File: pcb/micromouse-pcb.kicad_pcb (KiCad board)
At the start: 4 copper layers, 120 x 80 mm, 52 parts, among them J1 Conn_01x08, J1_MotorEncoder1 Conn_01x06, J2_MotorEncoder1 Conn_01x06, J3 Conn_01x08, J4 Conn_01x08, Q1 BS170, Q2 TEFT4300, Q3 BS170, Q4 TEFT4300, Q5 BS170, Q6 TEFT4300, Q7 BS170, Q8 TEFT4300, SW1 SW_SPDT, U1 Teensy_4.1, U2 L7805

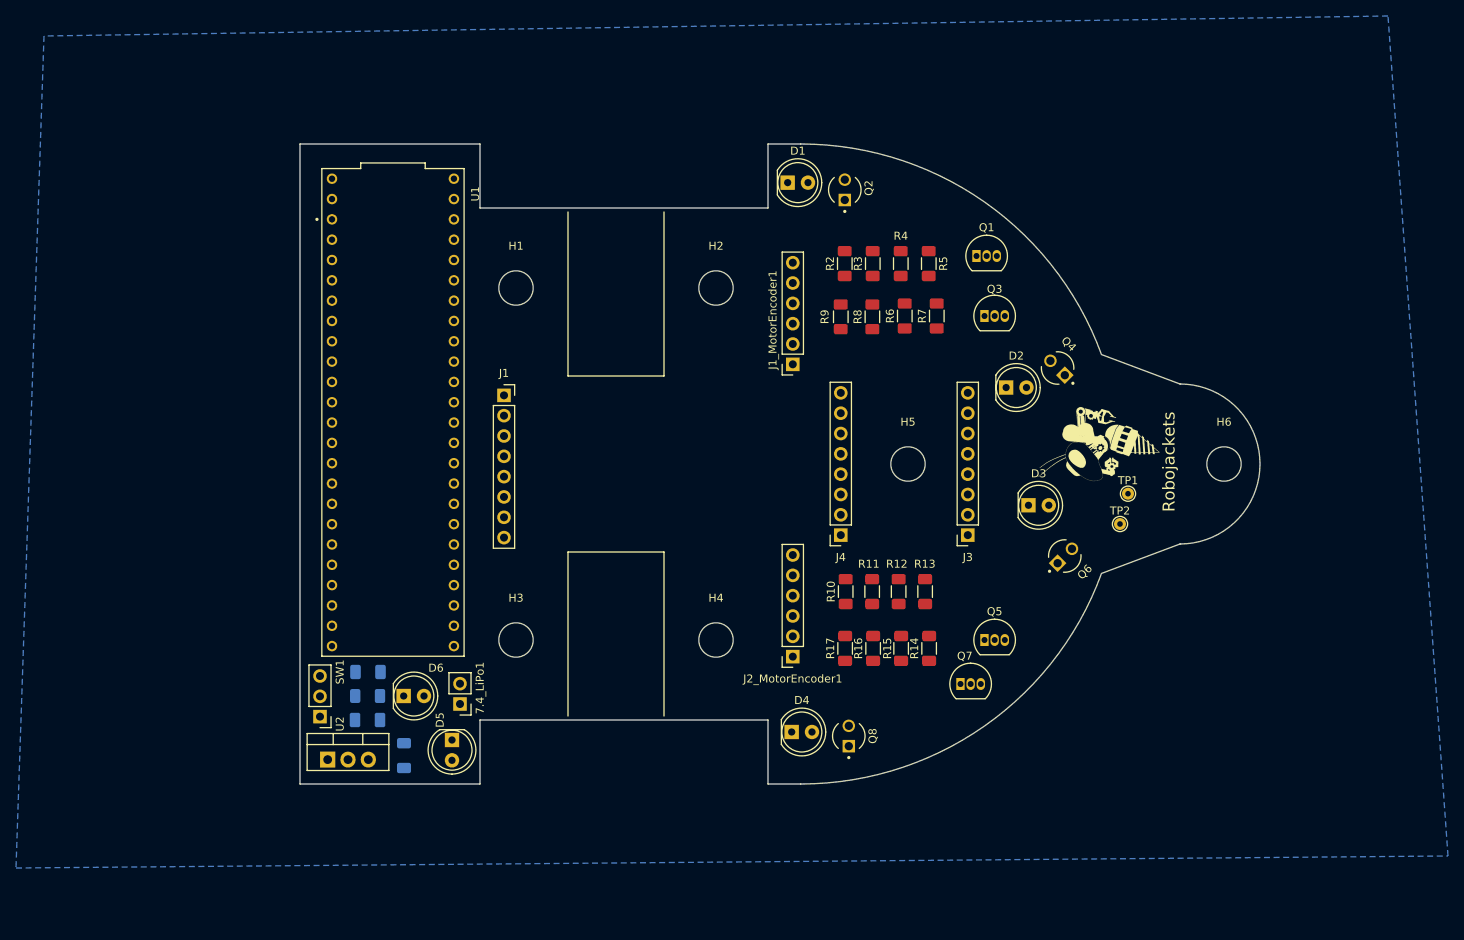
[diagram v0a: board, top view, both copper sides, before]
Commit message: Done placement
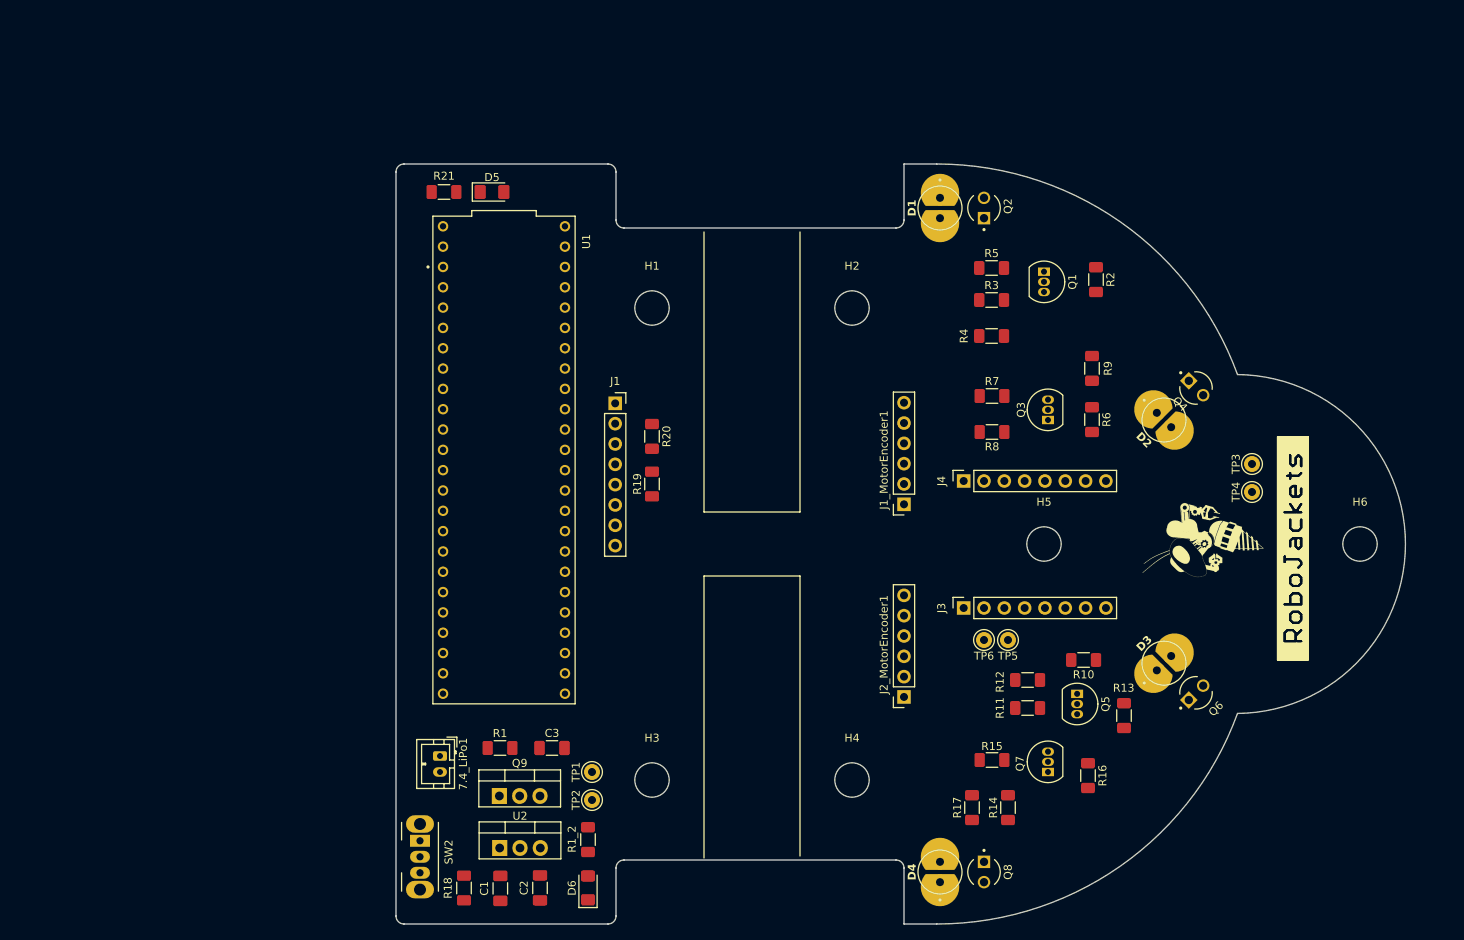
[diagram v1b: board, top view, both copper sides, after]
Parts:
- removed the ? at (122.5, 53.6)
- removed R1_1: R_US, Resistor_SMD:R_1206_3216Metric_Pad1.30x1.75mm_HandSolder
- removed SW1: SW_SPDT, Connector_PinHeader_2.54mm:PinHeader_1x03_P2.54mm_Vertical
- added ?: , micromouse:ROBOJACKETS, F.Cu at (141.0, 79.5)
- added ?: , micromouse:ROBOBUZZ_0.8X, F.Cu at (135.5, 65.6)
- added C3: C, Capacitor_SMD:C_1206_3216Metric_Pad1.33x1.80mm_HandSolder, F.Cu at (46.5, 90.5)
- added Q9: FQP27P06, Package_TO_SOT_THT:TO-220-3_Vertical, F.Cu at (39.9, 96.5)
- added R1: R_US, Resistor_SMD:R_1206_3216Metric_Pad1.30x1.75mm_HandSolder, F.Cu at (40.0, 90.5)
- added R18: R_US, Resistor_SMD:R_1206_3216Metric_Pad1.30x1.75mm_HandSolder, F.Cu at (35.5, 108.0)
- added R19: 4.7k, Resistor_SMD:R_1206_3216Metric_Pad1.30x1.75mm_HandSolder, F.Cu at (59.0, 57.5)
- added R20: 4.7k, Resistor_SMD:R_1206_3216Metric_Pad1.30x1.75mm_HandSolder, F.Cu at (59.0, 51.5)
- added R21: 1k, Resistor_SMD:R_1206_3216Metric_Pad1.30x1.75mm_HandSolder, F.Cu at (33.0, 21.0)
- added SW2: SW_SPDT, Button_Switch_THT:SW_Slide_SPDT_Angled_CK_OS102011MA1Q, F.Cu at (30.0, 102.1)
- added TP3: TestPoint, micromouse:TestPoint_THTPad_D2.0mm_Drill1.0mm, F.Cu at (134.0, 55.0)
- added TP4: TestPoint, micromouse:TestPoint_THTPad_D2.0mm_Drill1.0mm, F.Cu at (134.0, 58.5)
- added TP5: TestPoint, micromouse:TestPoint_THTPad_D2.0mm_Drill1.0mm, F.Cu at (103.5, 77.0)
- added TP6: TestPoint, micromouse:TestPoint_THTPad_D2.0mm_Drill1.0mm, F.Cu at (100.5, 77.0)
- 7.4_LiPo1: footprint Connector_PinHeader_2.54mm:PinHeader_1x02_P2.54mm_Vertical -> Connector_JST:JST_PH_B2B-PH-K_1x02_P2.00mm_Vertical
- C1, C2, R1_2: moved to F.Cu
- D1, D2, D3, D4: footprint micromouse:LED_D5.0mm_IR -> micromouse:DIO_SFH_4545_copy
- D5, D6: footprint LED_THT:LED_D5.0mm -> LED_SMD:LED_1206_3216Metric_Pad1.42x1.75mm_HandSolder
- R2: value R_US -> 100/75
- R3: value R_US -> 1.3k
- R4: value R_US -> 2k
- TP1, TP2: footprint TestPoint:TestPoint_THTPad_D1.5mm_Drill0.7mm -> micromouse:TestPoint_THTPad_D2.0mm_Drill1.0mm
- moved TP1 75.5 mm to (51.5, 93.5)
- moved TP2 74.5 mm to (51.5, 97.0)
- moved D5 68.7 mm to (39.0, 21.0), turned to 0 degrees
- moved C2 34.5 mm to (45.0, 108.0), turned to 90 degrees
- moved D6 33.3 mm to (51.0, 108.0), turned to 90 degrees
- moved R1_2 32.9 mm to (51.0, 102.0), turned to -90 degrees
- moved R9 32.1 mm to (114.0, 43.0), turned to -90 degrees
- moved R2 31.5 mm to (114.5, 31.9), turned to -90 degrees
- moved R16 31.2 mm to (113.5, 94.0), turned to -90 degrees
- moved R10 30.9 mm to (113.0, 79.5), turned to 180 degrees
- moved R13 29.3 mm to (118.0, 86.5)
- moved C1 26.8 mm to (40.0, 108.0), turned to -90 degrees
- moved R6 26.7 mm to (114.0, 49.5), turned to -90 degrees
- moved D3 26.0 mm to (123.0, 79.9), turned to 45 degrees
- moved D4 25.5 mm to (95.0, 106.0), turned to 90 degrees
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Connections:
- net M1_A renamed POW_M1_A
- net M1_B renamed POW_M1_B
- net M2_A renamed POW_M2_A
- net M2_B renamed POW_M2_B
- C2 pad 1: 5V -> GND
- C2 pad 2: GND -> 5V
- D5 pad 1: Net-(D5-K) -> GND
- D5 pad 2: 7.4V -> Net-(D5-A)
- J1_MotorEncoder1 pad 2: Signal M1_A -> ENC_M1_A
- J1_MotorEncoder1 pad 3: Signal M1_B -> ENC_M1_B
- J2_MotorEncoder1 pad 2: Signal M2_A -> ENC_M2_A
- J2_MotorEncoder1 pad 3: Signal M2_B -> ENC_M2_B
- J3 pad 2: unconnected-(J3-Pin_2-Pad2) -> Net-(J3-Pin_2)
- J4 pad 1: unconnected-(J4-Pin_1-Pad1) -> PWMA_6612
- J4 pad 7: unconnected-(J4-Pin_7-Pad7) -> PWMB_6612
- U1 pad 0: unconnected-(U1-RX1-Pad0) -> Net-(U1-RX1)
- U1 pad 10: Emitter 2 -> unconnected-(U1-CS1-Pad10)
- U1 pad 11: Emitter 3 -> PWMA_6612
- U1 pad 12: Emitter 4 -> PWMB_6612
- U1 pad 14: Signal M1_A -> unconnected-(U1-A0-Pad14)
- U1 pad 15: Signal M1_B -> unconnected-(U1-A1-Pad15)
- U1 pad 34: unconnected-(U1-RX8-Pad34) -> ENC_M1_A
- U1 pad 35: unconnected-(U1-TX8-Pad35) -> ENC_M1_B
- U1 pad 36: unconnected-(U1-CS2-Pad36) -> ENC_M2_A
- U1 pad 37: unconnected-(U1-CS3-Pad37) -> ENC_M2_B
- U1 pad 38: unconnected-(U1-A14-Pad38) -> Emitter 1
- U1 pad 39: unconnected-(U1-A15-Pad39) -> Emitter 2
- U1 pad 40: Signal M2_A -> Emitter 3
- U1 pad 41: Signal M2_B -> Emitter 4
- U1 pad 9: Emitter 1 -> unconnected-(U1-OUT1C-Pad9)
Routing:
- added copper zone on In1.Cu, net GND
- removed copper zone on B.Cu, net GND
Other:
- board size 120 x 80 mm -> 126.2 x 95 mm
- board text removed: "Robojackets"
